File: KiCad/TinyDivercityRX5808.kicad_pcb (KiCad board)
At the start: 2 copper layers, 52 x 34.5 mm, 28 parts, among them J1 Googles, J4 PROG, SW1 SW_DPST, U1 MAX4624, U2 ATTINY85-20SU, U3 MAX4625

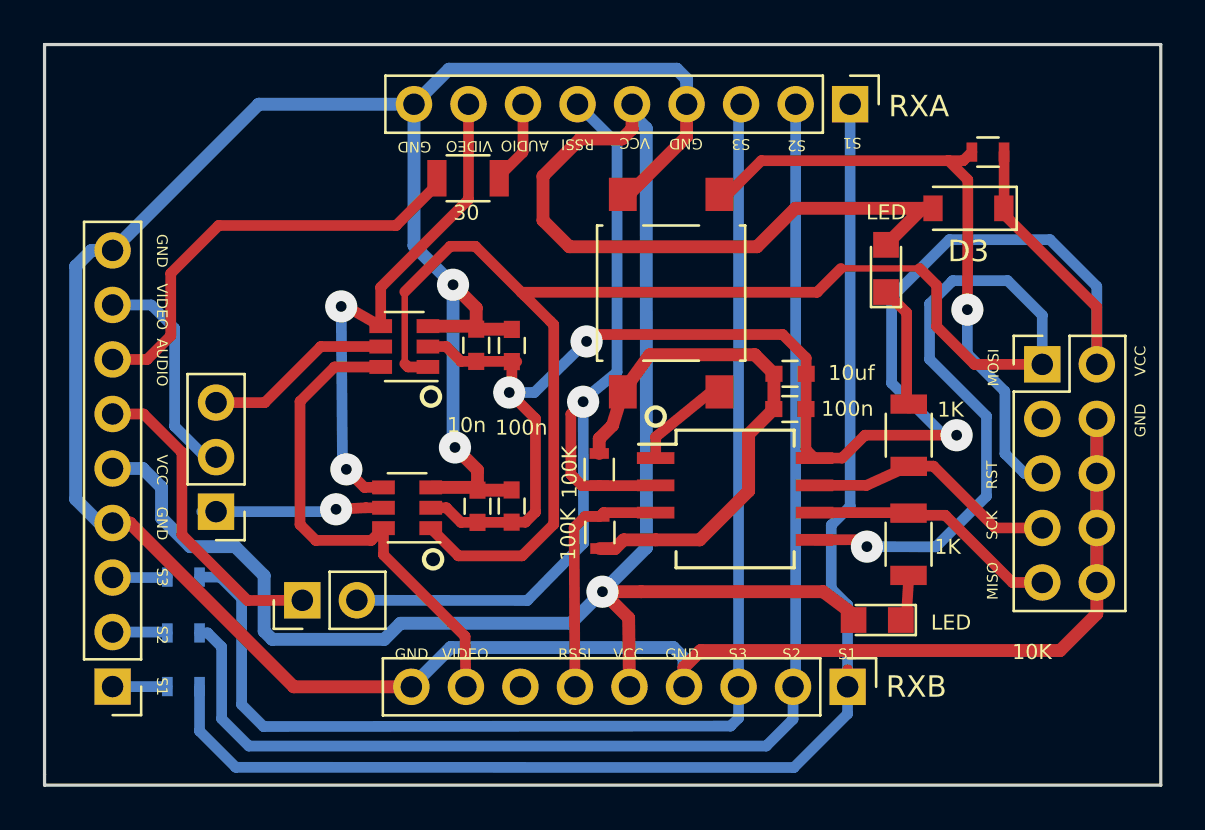
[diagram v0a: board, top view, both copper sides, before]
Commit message: First draft of final PCB
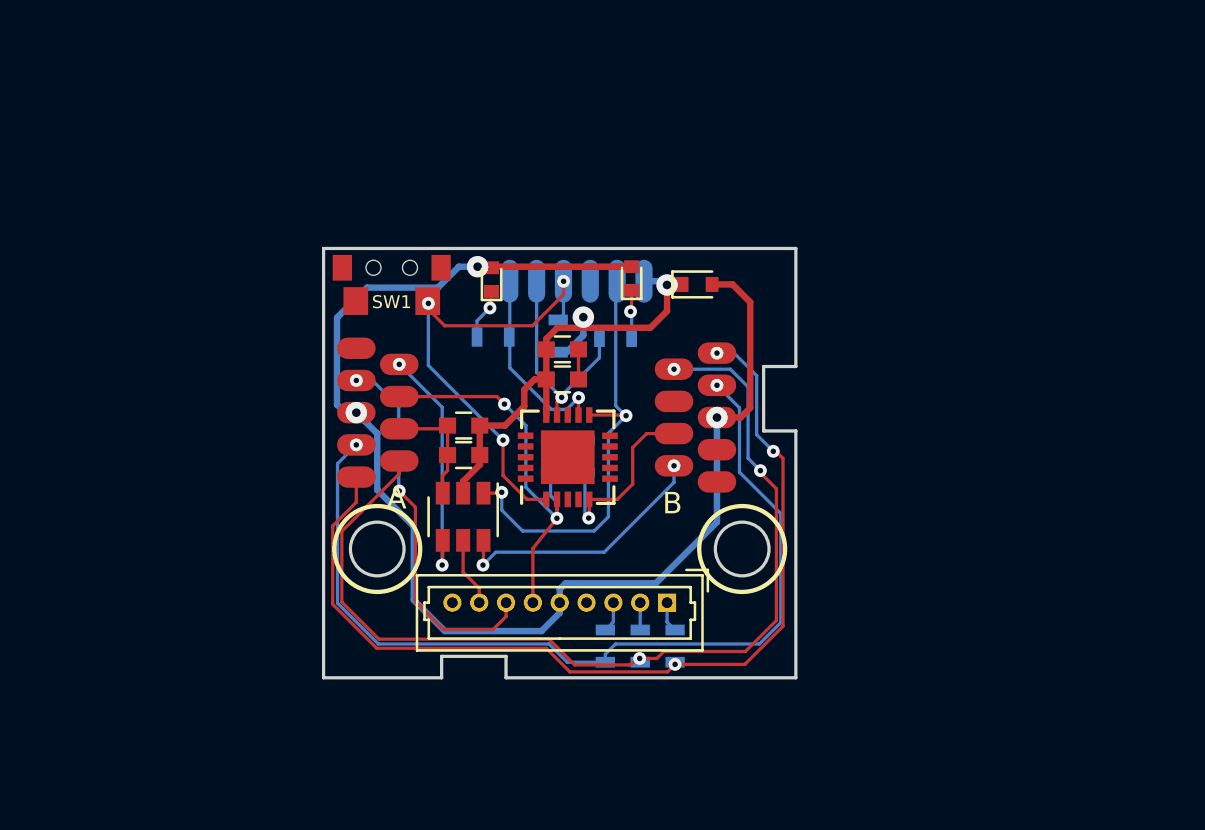
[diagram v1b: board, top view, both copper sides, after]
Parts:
- removed C5: 100n, Capacitors_SMD:C_0603
- removed C6: 10n, Capacitors_SMD:C_0603
- removed JP1: Jumper, Pin_Headers:Pin_Header_Straight_1x02_Pitch2.54mm
- removed JP2: Video4/5, Pin_Headers:Pin_Header_Straight_1x03_Pitch2.54mm
- removed RXA: RX_A, Pin_Headers:Pin_Header_Straight_1x09_Pitch2.54mm
- removed RXB: RX_B, Pin_Headers:Pin_Header_Straight_1x09_Pitch2.54mm
- removed U3: MAX4625, TO_SOT_Packages_SMD:SOT-23-6
- added J2: RX_A, KiCadCustomLibs:Pads_9pin_chess, F.Cu at (130.3, 99.7)
- added J3: RX_B, KiCadCustomLibs:Pads_9pin_chess, F.Cu at (147.1, 99.9)
- D1, D2: footprint LEDs:LED_0805 -> LEDs:LED_0402
- D3: footprint Diodes_SMD:D_SOD-123 -> Diodes_SMD:D_SOD-523
- J1: footprint Pin_Headers:Pin_Header_Straight_1x09_Pitch2.54mm -> Connectors_Molex:Molex_PicoBlade_53047-0910_09x1.25mm_Straight
- J4: value PROG -> Conn_01x06; footprint Pin_Headers:Pin_Header_Straight_2x05_Pitch2.54mm -> KiCadCustomLibs:Pads_prog_6pin1.25mm; moved to B.Cu
- R4, R5, R9: moved to B.Cu
- R6: footprint Resistors_SMD:R_1206 -> Resistors_SMD:R_0603; moved to B.Cu
- R7: value 30 -> 1K; footprint Resistors_SMD:R_1206 -> Resistors_SMD:R_0603; moved to B.Cu
- R8: value 1K -> 30; footprint Resistors_SMD:R_1206 -> Resistors_SMD:R_0603; moved to B.Cu
- SW1: value SW_DPST -> SW_Push; footprint Buttons_Switches_SMD:SW_SPST_B3S-1000 -> KiCadCustomLibs:Button_TS-018
- U2: value ATTINY85-20SU -> ATTINY85-20MU; footprint Housings_SOIC:SO-8_5.3x6.2mm_Pitch1.27mm -> Housings_DFN_QFN:QFN-20-1EP_4x4mm_Pitch0.5mm
- moved J1 26.1 mm to (144.8, 108.5)
- moved R8 24.2 mm to (132.3, 101.4), turned to 90 degrees
- moved D2 24.0 mm to (136.6, 93.5), turned to 90 degrees
- moved R3 23.0 mm to (145.2, 110.6), turned to 270 degrees
- moved J4 22.0 mm to (140.6, 93.6), turned to 180 degrees
- moved R9 21.8 mm to (139.7, 96.1), turned to 270 degrees
- moved R2 21.3 mm to (143.6, 110.6), turned to 270 degrees
- moved R1 19.9 mm to (141.9, 110.6), turned to 270 degrees
- moved C1 15.3 mm to (135.3, 101.7)
- moved R6 14.4 mm to (142.4, 96.2), turned to 0 degrees
- moved D3 13.1 mm to (146.2, 93.7), turned to 0 degrees
- moved SW1 13.1 mm to (132.0, 93.0), turned to 0 degrees
- moved D1 11.9 mm to (143.2, 93.5)
- moved C4 10.6 mm to (139.9, 98.2), turned to 180 degrees
- moved U1 8.39 mm to (135.3, 104.5), turned to 270 degrees
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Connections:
- J1 pad 6: /RSSI_G -> /RSSI_A
- J4 pad 1: /MOSI -> /PROG_PWR
- J4 pad 2: /PROG_PWR -> /MOSI
- J4 pad 3: Net-(J4-Pad3) -> GND
- J4 pad 4: GND -> /RST
- J4 pad 5: /RST -> /SCK
- J4 pad 6: GND -> /MISO
- R7 pad 1: /AUD_IN -> /MISO
- R7 pad 2: /AUD_OUT -> Net-(D2-Pad1)
- R8 pad 1: /MISO -> /AUD_IN
- R8 pad 2: Net-(D2-Pad1) -> /AUD_OUT
- U1 pad 5: Net-(JP2-Pad3) -> /VideoOut
- U2 pad 3: /RSSI_B -> (no net)
- U2 pad 4: GND -> (no net)
- U2 pad 5: /MOSI -> /RSSI_B
- U2 pad 6: /MISO -> (no net)
- U2 pad 7: /SCK -> (no net)
- U2 pad 8: /PROG_PWR -> GND
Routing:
- net GND: track 177.6 -> 6.99 mm, vias 2 -> 0
- net /MOSI: track 85.5 -> 20.6 mm, vias 1 -> 2
- net /PROG_PWR: track 79.6 -> 23.8 mm, vias 3 -> 2
- net VCC: track 101.6 -> 60.8 mm, vias 1 -> 3
- net /RSSI_A: track 41.7 -> 18.8 mm, vias 1 -> 2
- net Net-(J2-Pad1): track 64.3 -> 44.2 mm, vias 0 -> 3
- net Net-(J2-Pad3): track 60.9 -> 42.8 mm, vias 0 -> 2
- net Net-(J2-Pad2): track 62.0 -> 45.4 mm, vias 0 -> 3
- net /RSSI_G: track 14.7 -> 0.00 mm
- net /VideoA: track 23.9 -> 11.3 mm
- net /RST: track 34.2 -> 22.2 mm, vias 1 -> 3
- net /VideoB: track 23.7 -> 12.4 mm, vias 0 -> 2
- net Net-(JP2-Pad3): track 8.92 -> 0.00 mm
- net Net-(JP2-Pad1): track 8.84 -> 0.00 mm, vias 1 -> 0
- net /AUD_IN: track 20.5 -> 12.3 mm, vias 0 -> 1
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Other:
- board size 52 x 34.5 mm -> 22 x 20 mm
- net class Default: clearance 0.3 -> 0.1524; trace_width 0.5 -> 0.1524; via_dia 1.5 -> 0.6; via_drill 0.5 -> 0.254
- net class GND: clearance 0.3 -> 0.2; trace_width 0.6 -> 0.3; via_dia 1.5 -> 1; via_drill 0.5 -> 0.4
- net class VCC: clearance 0.3 -> 0.1524; trace_width 0.6 -> 0.3; via_dia 1.5 -> 1; via_drill 0.5 -> 0.4
- rule pad_to_mask_clearance: 0.15 -> 0.06
- rule trace_clearance: 0.3 -> 0.1524
- rule trace_min: 0.2 -> 0.1524
- rule via_min_drill: 0.3 -> 0.254
- board text added: "A"
- board text added: "B"
- board text added: "PROG"
- board text removed: "100K"
- board text removed: "100n"
- board text removed: "10K"
- board text removed: "10n"
- board text removed: "10uf"
- board text removed: "1K"
- board text removed: "30"
- board text removed: "AUDIO"
- board text removed: "GND"
- board text removed: "LED"
- board text removed: "MISO"
- board text removed: "MOSI"
- board text removed: "RSSI"
- board text removed: "RST"
- board text removed: "S1"
- board text removed: "S2"
- board text removed: "S3"
- board text removed: "SCK"
- board text removed: "VCC"
- board text removed: "VIDEO"
